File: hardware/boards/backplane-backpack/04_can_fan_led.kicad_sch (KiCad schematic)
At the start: 22 parts, among them J2 GND/CANL/CANH (TBD), J9 12V FAN (TBD), Q1 AO3407A, Q2 2N7002,215, U3 TCAN3413DR

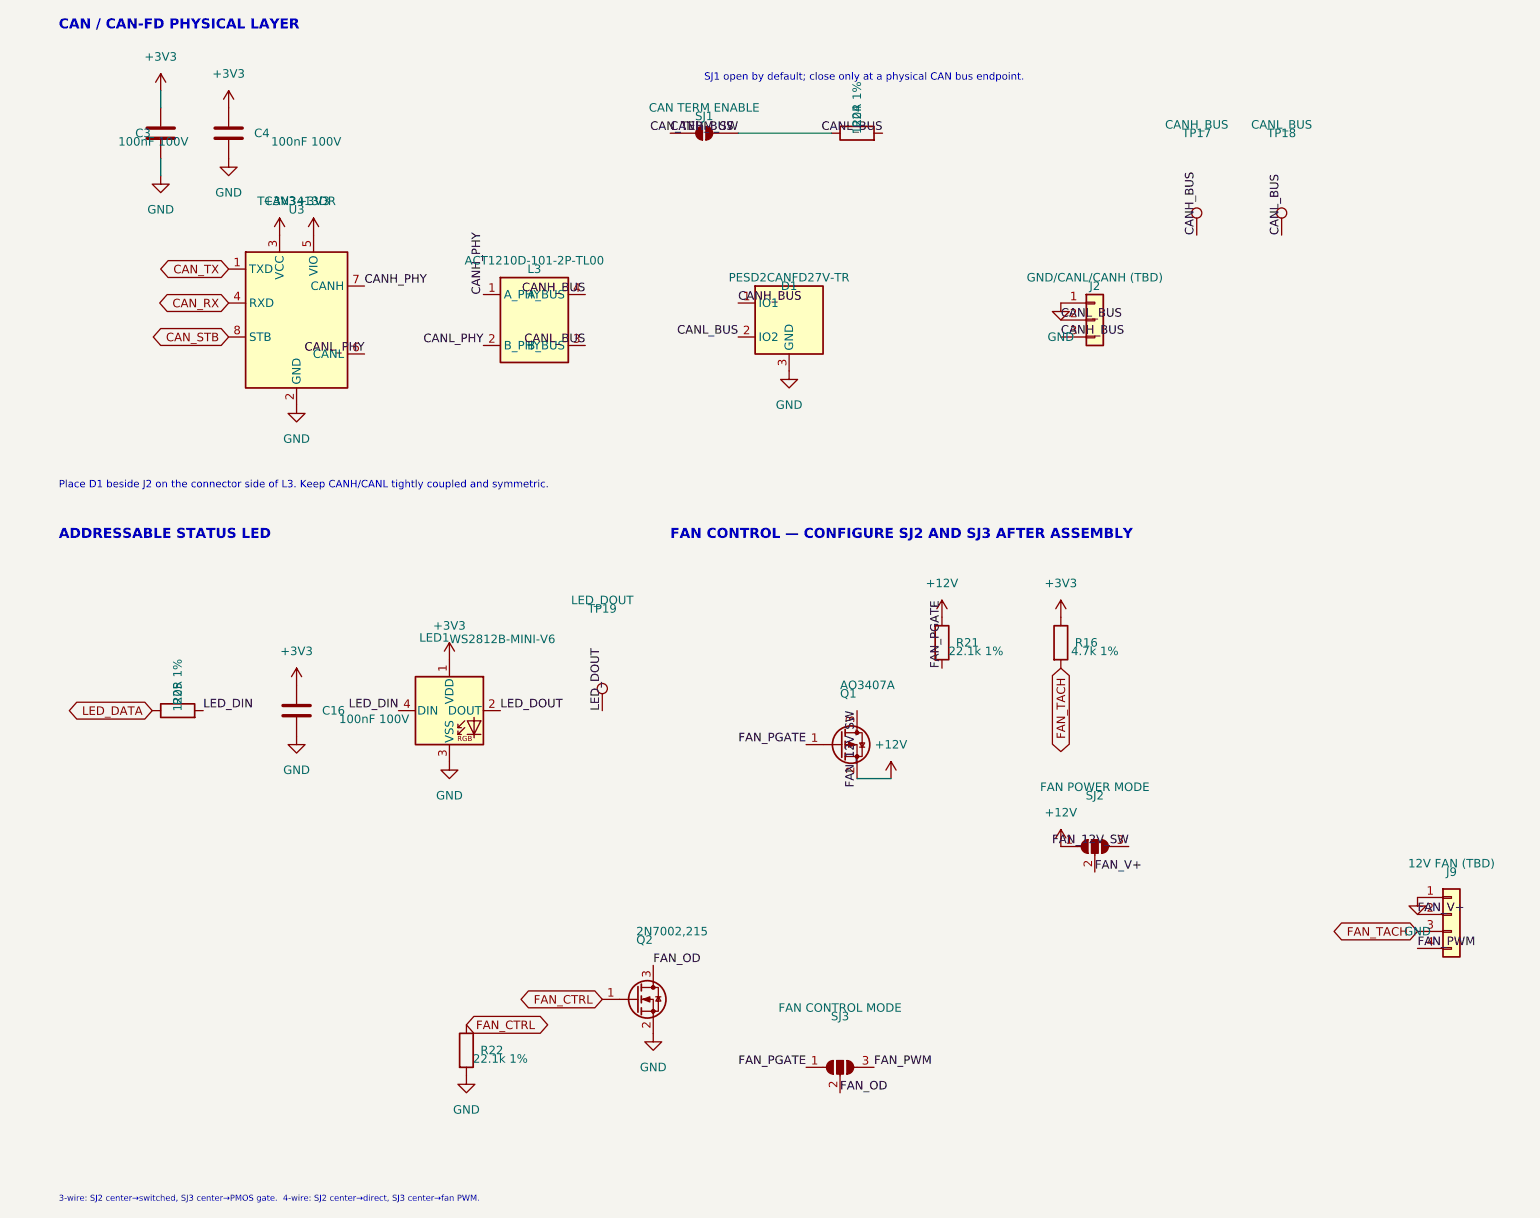
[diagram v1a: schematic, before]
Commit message: chore: checkpoint current board layout
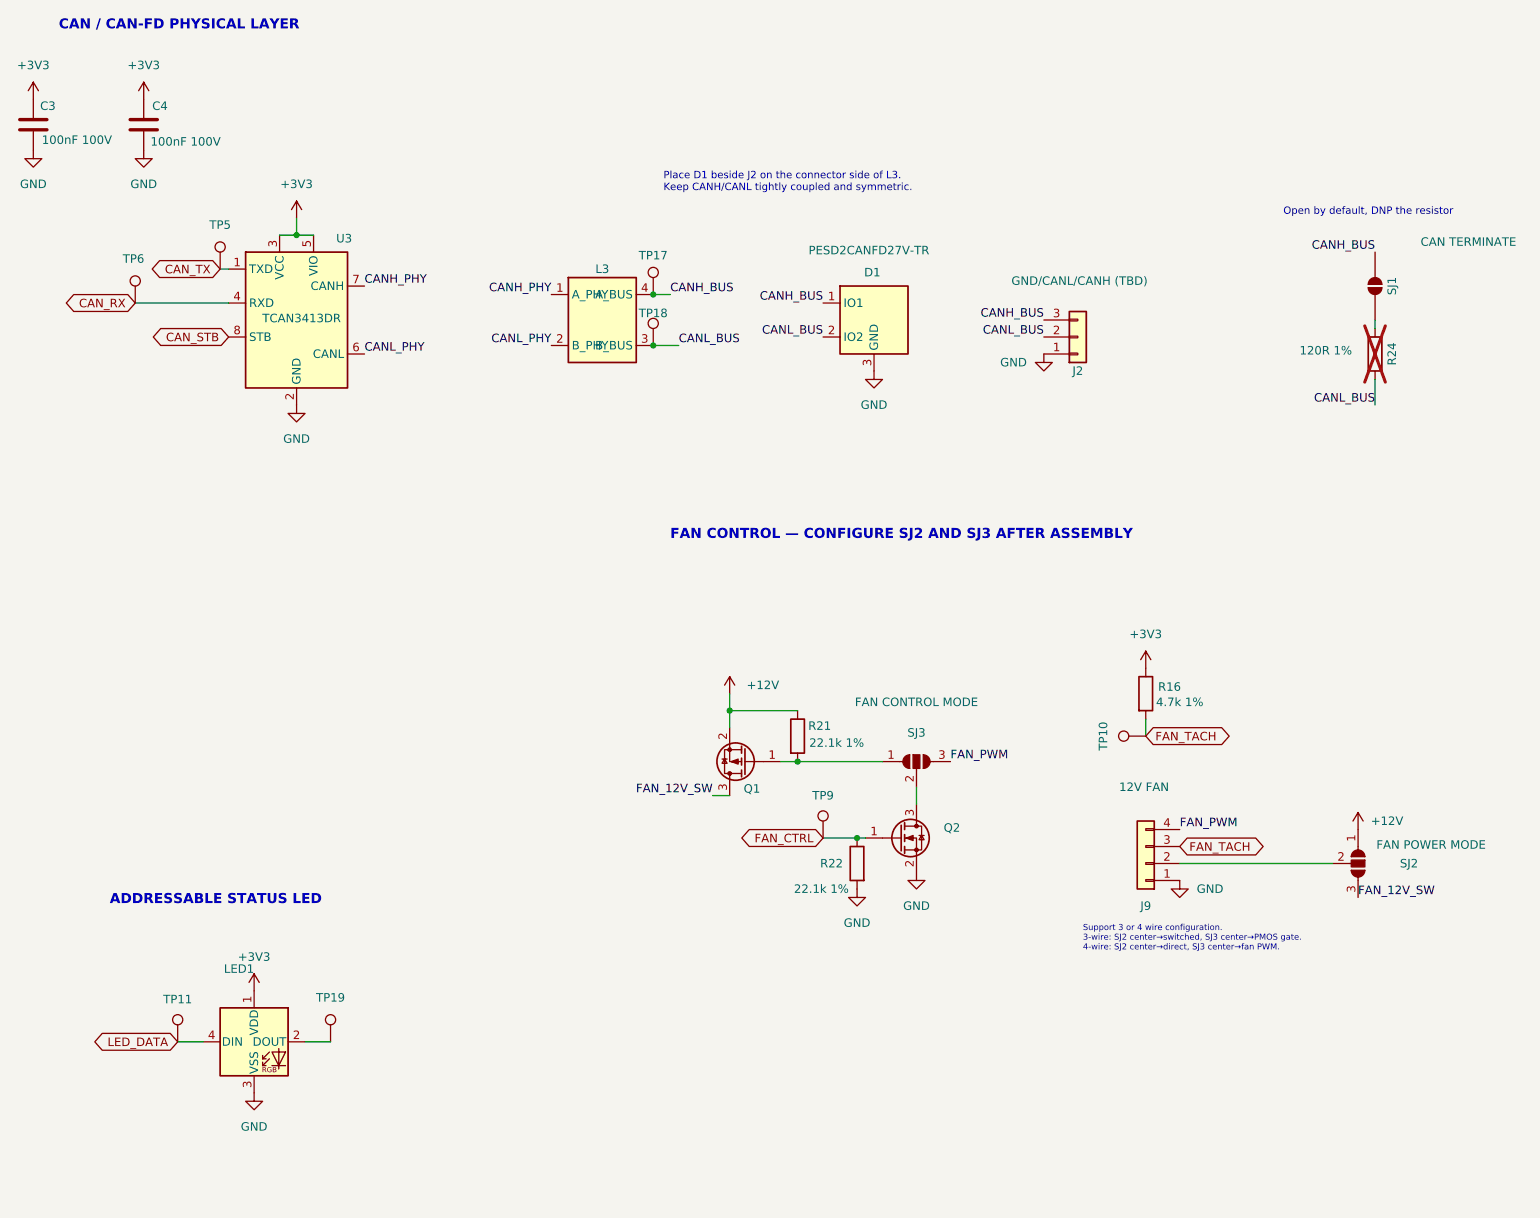
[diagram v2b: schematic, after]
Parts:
- removed C16: 100nF 100V, Capacitor_SMD:C_0603_1608Metric, symbol Device:C
- removed R25: 120R 1%, Resistor_SMD:R_0603_1608Metric, symbol Device:R
- added TP10: FAN_TACH, TestPoint:TestPoint_Pad_D1.5mm, symbol Connector:TestPoint
- added TP11: LED_DATA, TestPoint:TestPoint_Pad_D1.5mm, symbol Connector:TestPoint
- added TP5: CAN_TX, TestPoint:TestPoint_Pad_D1.5mm, symbol Connector:TestPoint
- added TP6: CAN_RX, TestPoint:TestPoint_Pad_D1.5mm, symbol Connector:TestPoint
- added TP9: FAN_CTRL, TestPoint:TestPoint_Pad_D1.5mm, symbol Connector:TestPoint
- J9: value 12V FAN (TBD) -> 12V FAN
- R24: now not fitted
- SJ1: value CAN TERM ENABLE -> CAN TERMINATE
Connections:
- net LED_DIN is gone; now on net LED_DATA: LED1.4 (DIN)
- net CAN_RX: now also TP6.1
- net CAN_TX: now also TP5.1
- net FAN_CTRL: now also TP9.1
- net FAN_TACH: now also TP10.1
- net LED_DATA: now also TP11.1
- net CAN_TERM_SW: no longer names the net of R24.1, SJ1.2 (B)
- net FAN_OD: no longer names the net of Q2.3 (D), SJ3.2 (C)
- net FAN_PGATE: no longer names the net of Q1.1 (G), R21.2, SJ3.1 (A)
- net FAN_V+: no longer names the net of J9.2 (Pin_2), SJ2.2 (C)
- net LED_DOUT: no longer names the net of LED1.2 (DOUT), TP19.1
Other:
- note added: "Open by default, DNP the resistor"
- note added: "Support 3 or 4 wire configuration. 3-wire: SJ2 center→switched, SJ3 center→PMOS gate. 4-wire: SJ2 center→direct, SJ3 center→fan PWM."
- note removed: "3-wire: SJ2 center→switched, SJ3 center→PMOS gate. 4-wire: SJ2 center→direct, SJ3 center→fan PWM."
- note removed: "SJ1 open by default; close only at a physical CAN bus endpoint."
- moved on the sheet: C3, C4, D1, J2, J9, L3, LED1, Q1, Q2, R16, R22, SJ2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
